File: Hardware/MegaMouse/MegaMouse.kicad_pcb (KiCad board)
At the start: 2 copper layers, 94 x 99 mm, 7 parts, among them J101 MotorL, J102 MotorR, U101 ATmega328P-A, U102 HDSP-7803

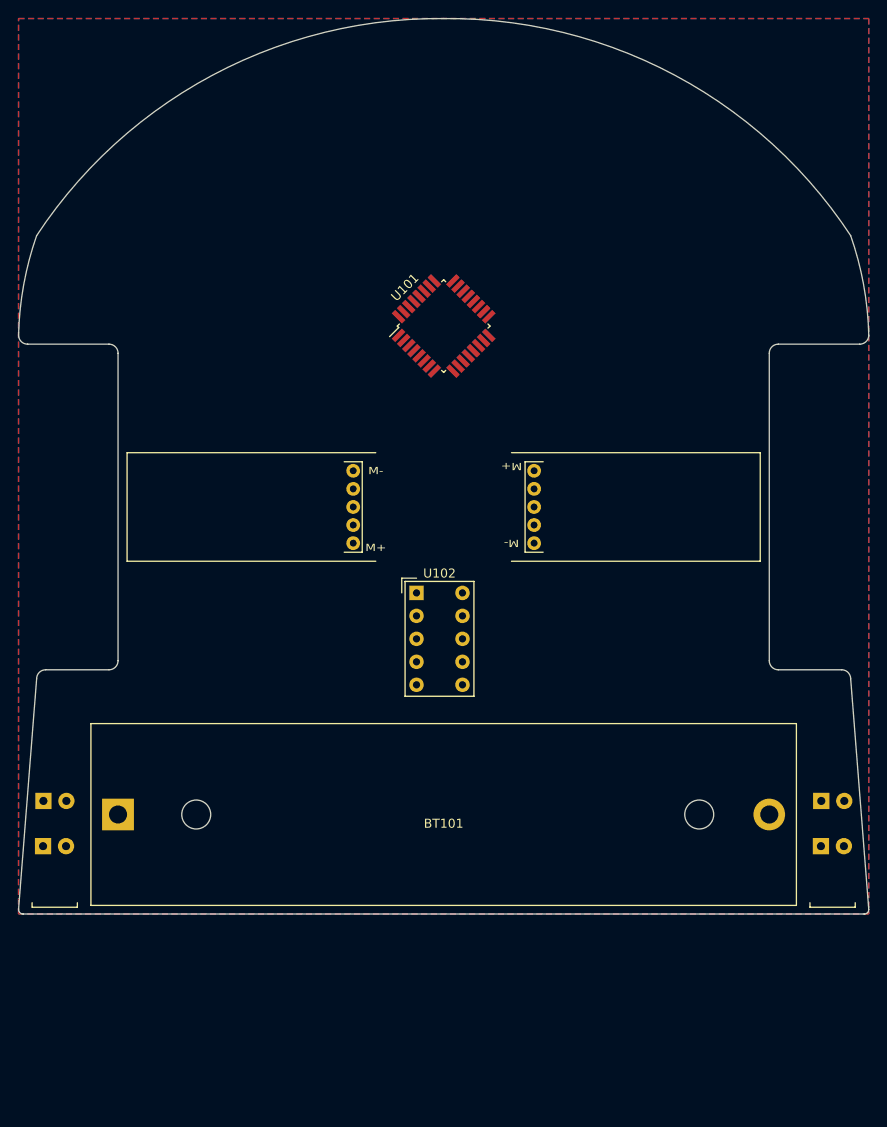
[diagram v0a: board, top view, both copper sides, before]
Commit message: Make awesome
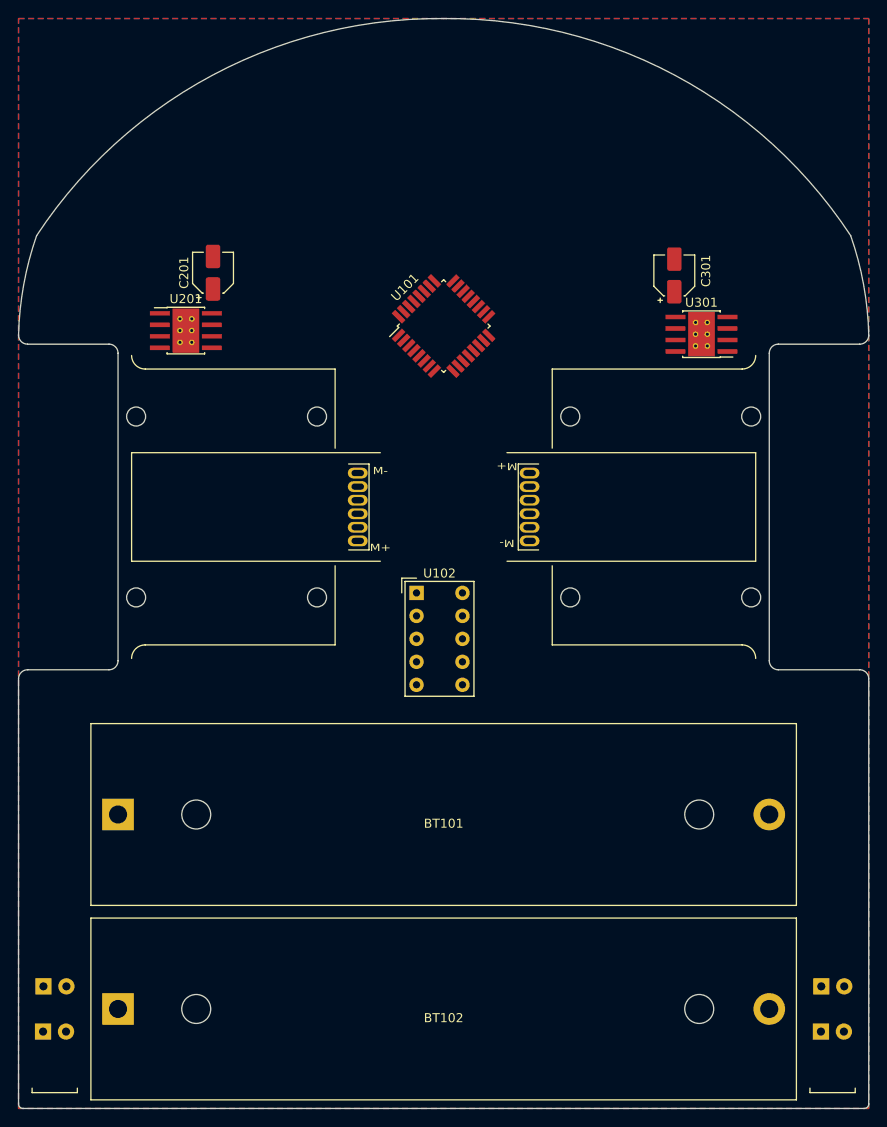
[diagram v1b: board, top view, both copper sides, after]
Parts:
- removed J101: MotorL, MegaMouse:MicroMotor
- removed J102: MotorR, MegaMouse:MicroMotor
- added BT102: Cell2, Battery:BatteryHolder_MPD_BH-18650-PC2, F.Cu at (-36.0, 55.5)
- added C201: 10uf, Capacitor_SMD:CP_Elec_4x3, F.Cu at (-25.5, -25.9)
- added C301: 10uf, Capacitor_SMD:CP_Elec_4x3, F.Cu at (25.5, -25.6)
- added J201: Motor, MegaMouse:MicroMotor, F.Cu at (-9.50, 0.00)
- added J301: Motor, MegaMouse:MicroMotor, F.Cu at (9.50, 0.00)
- added U201: DRV8871DDA, Package_SO:Texas_HTSOP-8-1EP_3.9x4.9mm_P1.27mm_EP2.95x4.9mm_Mask2.4x3.1mm_ThermalVias, F.Cu at (-28.5, -19.5)
- added U301: DRV8871DDA, Package_SO:Texas_HTSOP-8-1EP_3.9x4.9mm_P1.27mm_EP2.95x4.9mm_Mask2.4x3.1mm_ThermalVias, F.Cu at (28.5, -19.1)
- BT101: value Battery_Cell -> Cell1
- moved D101 20.5 mm to (-43.0, 58.0)
- moved D102 20.5 mm to (43.0, 58.0)
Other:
- board size 94 x 99 mm -> 94 x 120.5 mm
